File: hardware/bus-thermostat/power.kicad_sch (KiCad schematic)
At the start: 19 parts, among them SW1 SW_Push, U2 L7806, U3 LM7906_TO220, U4 MAX6420UK33+T, U5 NCP565D2T33R4G, U6 TLV9301IDCK

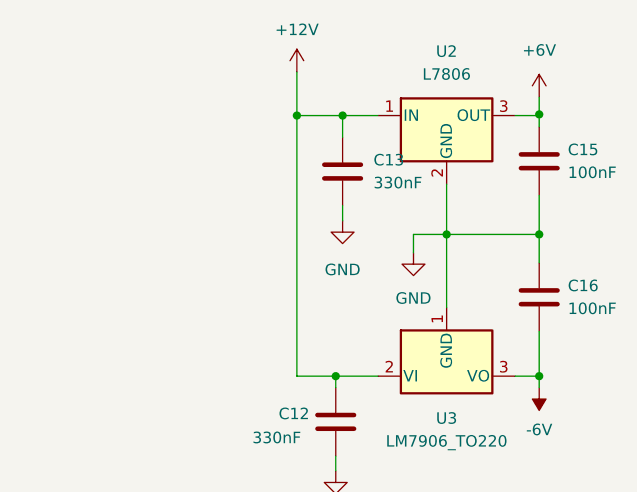
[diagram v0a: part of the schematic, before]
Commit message: First rev of thermostat firmware
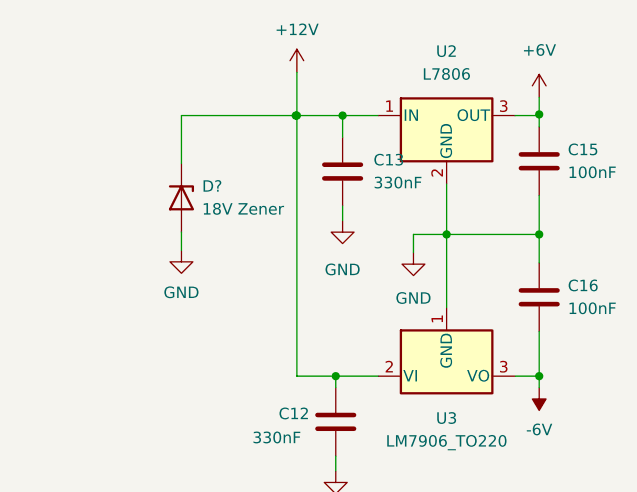
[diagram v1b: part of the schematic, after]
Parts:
- added D?: 18V Zener, symbol Device:D_Zener
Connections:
- net GND: now also D?.2 (A)
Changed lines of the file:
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@@
   (junction (at 78.105 53.213) (diameter 0) (color 0 0 0 0)
   )
+  (junction (at 51.054 40.005) (diameter 0) (color 0 0 0 0)
+  )
   (junction (at 173.355 44.196) (diameter 0) (color 0 0 0 0)
   )
@@
     (stroke (width 0) (type default) (color 0 0 0 0))
   )
+  (wire (pts (xy 38.354 52.959) (xy 38.354 54.991))
+    (stroke (width 0) (type default) (color 0 0 0 0))
+  )
   (wire (pts (xy 210.82 111.506) (xy 210.82 93.091))
     (stroke (width 0) (type default) (color 0 0 0 0))
@@
     (stroke (width 0) (type default) (color 0 0 0 0))
   )
+  (wire (pts (xy 38.354 40.005) (xy 51.054 40.005))
+    (stroke (width 0) (type default) (color 0 0 0 0))
+  )
   (wire (pts (xy 240.665 54.356) (xy 240.665 58.166))
     (stroke (width 0) (type default) (color 0 0 0 0))
@@
   )
   (wire (pts (xy 255.905 54.356) (xy 255.905 58.166))
+    (stroke (width 0) (type default) (color 0 0 0 0))
+  )
+  (wire (pts (xy 38.354 40.005) (xy 38.354 45.339))
     (stroke (width 0) (type default) (color 0 0 0 0))
   )
@@
     (pin "1")
     (pin "2")
+  )
+  (symbol (lib_name "GND_2") (lib_id "power:GND") (at 38.354 54.991 0) (unit 1)
+    (in_bom yes) (on_board yes) (fields_autoplaced)
+    (property "Reference" "#PWR?" (id 0) (at 38.354 61.341 0)
+      (effects (font (size 1.27 1.27)) hide)
+    )
+    (property "Value" "GND" (id 1) (at 38.354 59.69 0))
+    (property "Footprint" "" (id 2) (at 38.354 54.991 0)
+      (effects (font (size 1.27 1.27)) hide)
+    )
+    (property "Datasheet" "" (id 3) (at 38.354 54.991 0)
+      (effects (font (size 1.27 1.27)) hide)
+    )
+    (pin "1")
   )
   (symbol (lib_id "Device:R") (at 173.99 84.836 0) (unit 1)
@@
     (pin "1")
   )
+  (symbol (lib_id "Device:D_Zener") (at 38.354 49.149 270) (unit 1)
+    (in_bom yes) (on_board yes) (fields_autoplaced)
+    (property "Reference" "D?" (id 0) (at 40.64 47.8789 90)
+      (effects (font (size 1.27 1.27)) (justify left))
+    )
+    (property "Value" "18V Zener" (id 1) (at 40.64 50.4189 90)
+      (effects (font (size 1.27 1.27)) (justify left))
+    )
+    (property "Footprint" "" (id 2) (at 38.354 49.149 0)
+      (effects (font (size 1.27 1.27)) hide)
+    )
+    (property "Datasheet" "~" (id 3) (at 38.354 49.149 0)
+      (effects (font (size 1.27 1.27)) hide)
+    )
+    (pin "1")
+    (pin "2")
+  )
   (symbol (lib_id "power:GND") (at 74.422 161.671 0) (mirror y) (unit 1)
